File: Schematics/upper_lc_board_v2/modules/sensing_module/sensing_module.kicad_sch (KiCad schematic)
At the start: 19 parts, among them J5 HALL-1, U7 ADC_ADS131M04IPWR

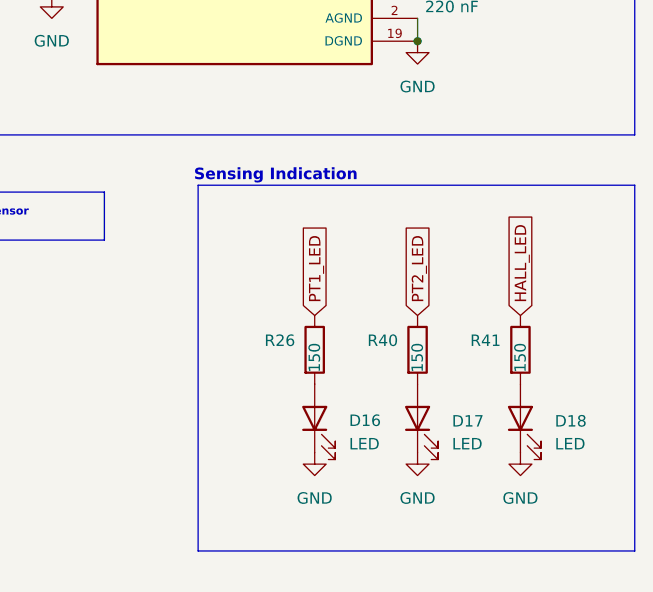
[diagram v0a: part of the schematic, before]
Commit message: review work
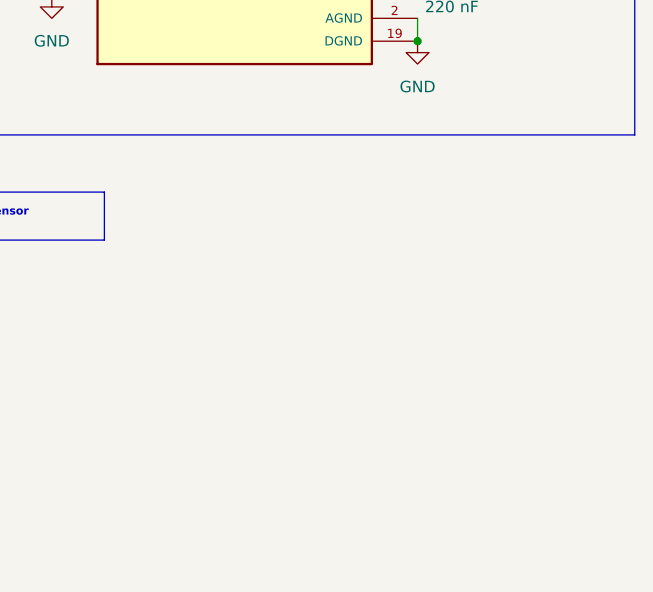
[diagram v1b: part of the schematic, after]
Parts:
- removed D16, D17, D18: LED, LED_SMD:LED_0603_1608Metric, symbol Device:LED
- removed R26, R40, R41: 150, Resistor_SMD:R_0603_1608Metric, symbol Device:R
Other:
- note removed: "Sensing Indication"
